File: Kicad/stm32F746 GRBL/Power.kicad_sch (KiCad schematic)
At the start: 1 part, among them J13 Screw_Terminal_01x04

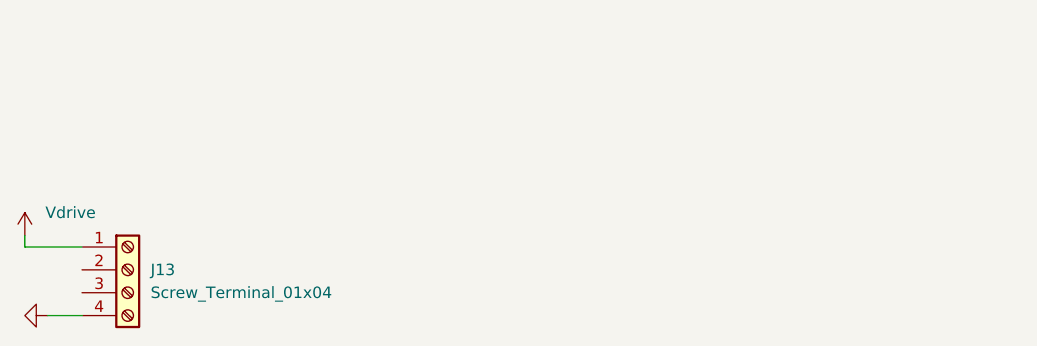
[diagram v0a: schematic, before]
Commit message: wip
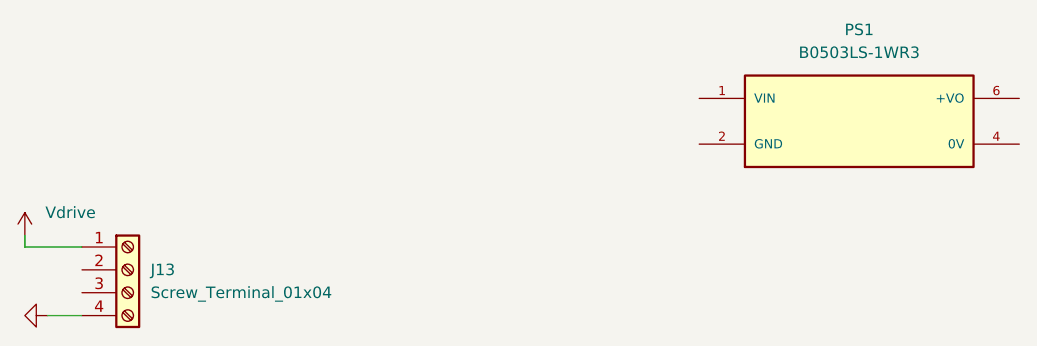
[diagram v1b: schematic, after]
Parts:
- added PS1: B0503LS-1WR3, stm32F746 GRBL:CONV_B0503LS-1WR3, symbol B0503LS-1WR3:B0503LS-1WR3
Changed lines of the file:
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@@
+    )
+  )
+  (symbol (lib_id "B0503LS-1WR3:B0503LS-1WR3") (at 153.67 69.85 0) (unit 1)
+    (in_bom yes) (on_board yes) (dnp no) (fields_autoplaced)
+    (property "Reference" "PS1" (at 153.67 59.69 0)
+      (effects (font (size 1.27 1.27)))
+    )
+    (property "Value" "B0503LS-1WR3" (at 153.67 62.23 0)
+      (effects (font (size 1.27 1.27)))
+    )
+    (property "Footprint" "stm32F746 GRBL:CONV_B0503LS-1WR3" (at 153.67 69.85 0)
+      (effects (font (size 1.27 1.27)) (justify bottom) hide)
+    )
+    (property "Datasheet" "" (at 153.67 69.85 0)
+      (effects (font (size 1.27 1.27)) hide)
+    )
+    (property "MF" "MORNSUN" (at 153.67 69.85 0)
+      (effects (font (size 1.27 1.27)) (justify bottom) hide)
+    )
+    (property "MAXIMUM_PACKAGE_HEIGHT" "10.41 mm" (at 153.67 69.85 0)
+      (effects (font (size 1.27 1.27)) (justify bottom) hide)
+    )
+    (property "Package" "SIP-4-4 MORNSUN" (at 153.67 69.85 0)
+      (effects (font (size 1.27 1.27)) (justify bottom) hide)
+    )
+    (property "Price" "None" (at 153.67 69.85 0)
+      (effects (font (size 1.27 1.27)) (justify bottom) hide)
+    )
+    (property "Check_prices" "https://www.snapeda.com/parts/B0503LS-1WR3/MORNSUN/view-part/?ref=eda" (at 153.67 69.85 0)
+      (effects (font (size 1.27 1.27)) (justify bottom) hide)
+    )
+    (property "STANDARD" "Manufacturer Recommendations" (at 153.67 69.85 0)
+      (effects (font (size 1.27 1.27)) (justify bottom) hide)
+    )
+    (property "PARTREV" "2019.10.15-A/5" (at 153.67 69.85 0)
+      (effects (font (size 1.27 1.27)) (justify bottom) hide)
+    )
+    (property "SnapEDA_Link" "https://www.snapeda.com/parts/B0503LS-1WR3/MORNSUN/view-part/?ref=snap" (at 153.67 69.85 0)
+      (effects (font (size 1.27 1.27)) (justify bottom) hide)
+    )
+    (property "MP" "B0503LS-1WR3" (at 153.67 69.85 0)
+      (effects (font (size 1.27 1.27)) (justify bottom) hide)
+    )
+    (property "Description" "\nIsolated Module DC DC Converter 1 Output 3.3V - - - 303mA 4.5V - 5.5V Input\n" (at 153.67 69.85 0)
+      (effects (font (size 1.27 1.27)) (justify bottom) hide)
+    )
+    (property "Availability" "In Stock" (at 153.67 69.85 0)
+      (effects (font (size 1.27 1.27)) (justify bottom) hide)
+    )
+    (property "MANUFACTURER" "Mornsun" (at 153.67 69.85 0)
+      (effects (font (size 1.27 1.27)) (justify bottom) hide)
+    )
+    (pin "2")
+    (pin "6")
+    (pin "1")
+    (pin "4")
+    (instances
+      (project "stm32F746 GRBL"
+        (path "/2c79a78e-687a-4954-b7b9-175bc3470bd7/cfe63f02-1987-4919-8e32-0515eff710ca"
+          (reference "PS1") (unit 1)
+        )
+      )
     )
   )

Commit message: wip Kicad
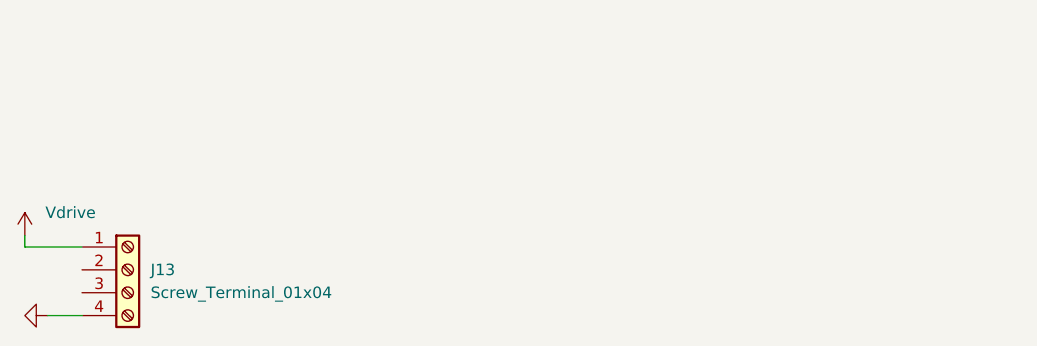
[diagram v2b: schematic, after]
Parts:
- removed PS1: B0503LS-1WR3, stm32F746 GRBL:CONV_B0503LS-1WR3, symbol B0503LS-1WR3:B0503LS-1WR3
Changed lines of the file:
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@@
-    )
-  )
-  (symbol (lib_id "B0503LS-1WR3:B0503LS-1WR3") (at 153.67 69.85 0) (unit 1)
-    (in_bom yes) (on_board yes) (dnp no) (fields_autoplaced)
-    (property "Reference" "PS1" (at 153.67 59.69 0)
-      (effects (font (size 1.27 1.27)))
-    )
-    (property "Value" "B0503LS-1WR3" (at 153.67 62.23 0)
-      (effects (font (size 1.27 1.27)))
-    )
-    (property "Footprint" "stm32F746 GRBL:CONV_B0503LS-1WR3" (at 153.67 69.85 0)
-      (effects (font (size 1.27 1.27)) (justify bottom) hide)
-    )
-    (property "Datasheet" "" (at 153.67 69.85 0)
-      (effects (font (size 1.27 1.27)) hide)
-    )
-    (property "MF" "MORNSUN" (at 153.67 69.85 0)
-      (effects (font (size 1.27 1.27)) (justify bottom) hide)
-    )
-    (property "MAXIMUM_PACKAGE_HEIGHT" "10.41 mm" (at 153.67 69.85 0)
-      (effects (font (size 1.27 1.27)) (justify bottom) hide)
-    )
-    (property "Package" "SIP-4-4 MORNSUN" (at 153.67 69.85 0)
-      (effects (font (size 1.27 1.27)) (justify bottom) hide)
-    )
-    (property "Price" "None" (at 153.67 69.85 0)
-      (effects (font (size 1.27 1.27)) (justify bottom) hide)
-    )
-    (property "Check_prices" "https://www.snapeda.com/parts/B0503LS-1WR3/MORNSUN/view-part/?ref=eda" (at 153.67 69.85 0)
-      (effects (font (size 1.27 1.27)) (justify bottom) hide)
-    )
-    (property "STANDARD" "Manufacturer Recommendations" (at 153.67 69.85 0)
-      (effects (font (size 1.27 1.27)) (justify bottom) hide)
-    )
-    (property "PARTREV" "2019.10.15-A/5" (at 153.67 69.85 0)
-      (effects (font (size 1.27 1.27)) (justify bottom) hide)
-    )
-    (property "SnapEDA_Link" "https://www.snapeda.com/parts/B0503LS-1WR3/MORNSUN/view-part/?ref=snap" (at 153.67 69.85 0)
-      (effects (font (size 1.27 1.27)) (justify bottom) hide)
-    )
-    (property "MP" "B0503LS-1WR3" (at 153.67 69.85 0)
-      (effects (font (size 1.27 1.27)) (justify bottom) hide)
-    )
-    (property "Description" "\nIsolated Module DC DC Converter 1 Output 3.3V - - - 303mA 4.5V - 5.5V Input\n" (at 153.67 69.85 0)
-      (effects (font (size 1.27 1.27)) (justify bottom) hide)
-    )
-    (property "Availability" "In Stock" (at 153.67 69.85 0)
-      (effects (font (size 1.27 1.27)) (justify bottom) hide)
-    )
-    (property "MANUFACTURER" "Mornsun" (at 153.67 69.85 0)
-      (effects (font (size 1.27 1.27)) (justify bottom) hide)
-    )
-    (pin "2")
-    (pin "6")
-    (pin "1")
-    (pin "4")
-    (instances
-      (project "stm32F746 GRBL"
-        (path "/2c79a78e-687a-4954-b7b9-175bc3470bd7/cfe63f02-1987-4919-8e32-0515eff710ca"
-          (reference "PS1") (unit 1)
-        )
-      )
     )
   )
